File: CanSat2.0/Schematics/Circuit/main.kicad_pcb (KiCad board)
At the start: 2 copper layers, 67.1 x 67.1 mm, 36 parts, among them J1 Center connector, J2 Middle connector, P1 CONN_2, P15 CONN_2, P2 CONN_2, P3 CONN_2, P4 CONN_2, SW7 SW_DIP_x01, U2 O2, U4 mg812_gas_sensor, U5 AD8572, U6 SP3_gas_sensor, U7 LMC662

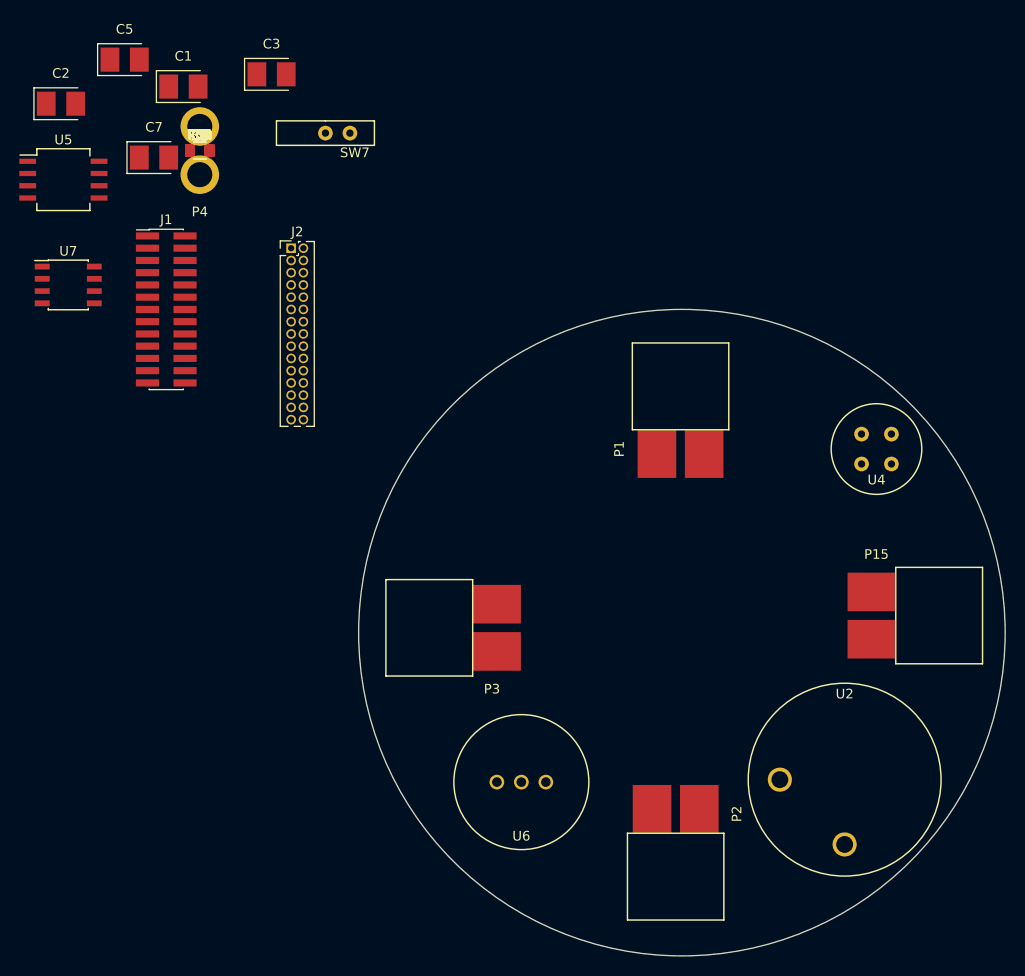
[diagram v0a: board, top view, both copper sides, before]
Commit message: PCBs
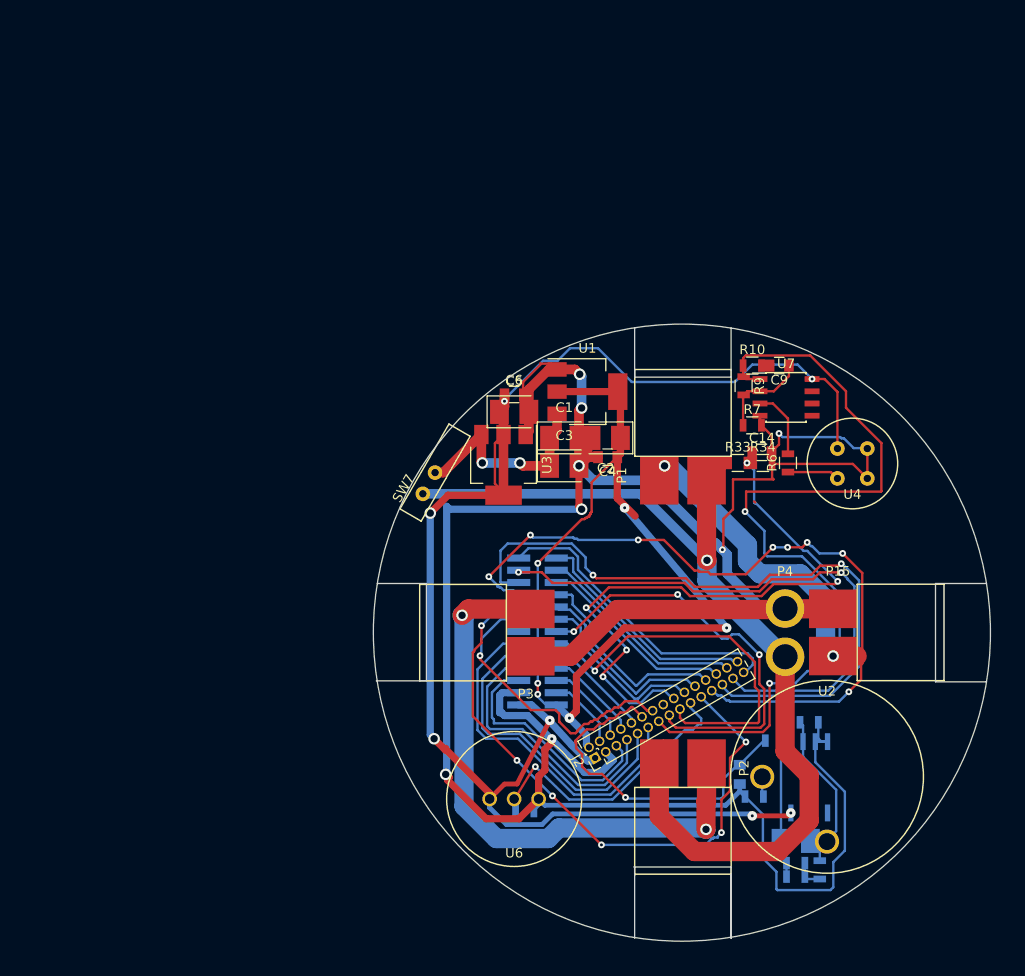
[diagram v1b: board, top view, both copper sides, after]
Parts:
- added U1: LD1117S33TR_SOT223, TO_SOT_Packages_SMD:SOT-223-3_TabPin2, F.Cu at (40.2, 25.0)
- added U3: LD1117S50TR_SOT223, TO_SOT_Packages_SMD:SOT-223-3_TabPin2, F.Cu at (31.5, 32.6)
- C7, C8, J1, R1, R2, R3, R4, R5, R8, TH1, U5: moved to B.Cu
- moved U5 99.1 mm to (63.2, 65.0), turned to 270 degrees
- moved R2 98.5 mm to (64.3, 74.6), turned to 270 degrees
- moved R4 97.4 mm to (61.8, 75.3), turned to 180 degrees
- moved C7 97.2 mm to (61.8, 71.6)
- moved TH1 96.3 mm to (61.8, 73.9)
- moved R1 88.3 mm to (57.5, 67.0)
- moved R3 86.7 mm to (63.2, 59.3), turned to 180 degrees
- moved C8 85.6 mm to (56.0, 64.7), turned to 270 degrees
- moved R5 85.4 mm to (59.6, 61.2), turned to 180 degrees
- moved P4 78.6 mm to (60.7, 50.0), turned to 180 degrees
- moved R8 76.3 mm to (33.7, 68.5)
- moved U7 75.3 mm to (60.8, 25.6)
- moved R6 69.1 mm to (61.0, 32.4), turned to 90 degrees
- moved R34 66.8 mm to (58.4, 32.4)
- moved C2 66.3 mm to (42.1, 29.8), turned to 180 degrees
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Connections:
- J1 pad 13: (no net) -> Net-(J1-Pad13)
- J2 pad 16: (no net) -> Net-(J2-Pad16)
- U5 pad 5: (no net) -> Net-(U5-Pad5)
- U5 pad 6: (no net) -> Net-(U5-Pad6)
- U5 pad 7: (no net) -> Net-(U5-Pad7)
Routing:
- net GND: track 0.00 -> 293.9 mm, vias 0 -> 8
- net +5V: track 0.00 -> 161.0 mm, vias 0 -> 7
- net +BATT: track 0.00 -> 99.1 mm, vias 0 -> 1
- net +3V3: track 0.00 -> 97.0 mm, vias 0 -> 6
- net /CO2: track 0.00 -> 92.0 mm, vias 0 -> 2
- net /FC_PWM_6: track 0.00 -> 71.8 mm, vias 0 -> 2
- net /V_READ: track 0.00 -> 66.5 mm, vias 0 -> 5
- net /RFM_SS: track 0.00 -> 63.5 mm, vias 0 -> 6
- net Net-(P1-Pad2): track 0.00 -> 61.2 mm, vias 0 -> 3
- net Net-(P2-Pad2): track 0.00 -> 61.1 mm, vias 0 -> 2
- net /FC_PWM_4: track 0.00 -> 59.8 mm, vias 0 -> 2
- net /FC_PWM_8: track 0.00 -> 49.7 mm, vias 0 -> 7
- net /SDA: track 0.00 -> 43.9 mm, vias 0 -> 3
- net /SERVO: track 0.00 -> 40.2 mm, vias 0 -> 1
- net /MISO: track 0.00 -> 36.8 mm
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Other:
- board size 67.1 x 67.1 mm -> 64 x 64 mm
